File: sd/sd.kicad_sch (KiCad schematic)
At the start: 34 parts, among them J1 Micro_SD_Card_Det2, J3 STM32WORLD_BOARD, J4 STM32WORLD_CONNECTOR_1, J5 STM32WORLD_CONNECTOR_2

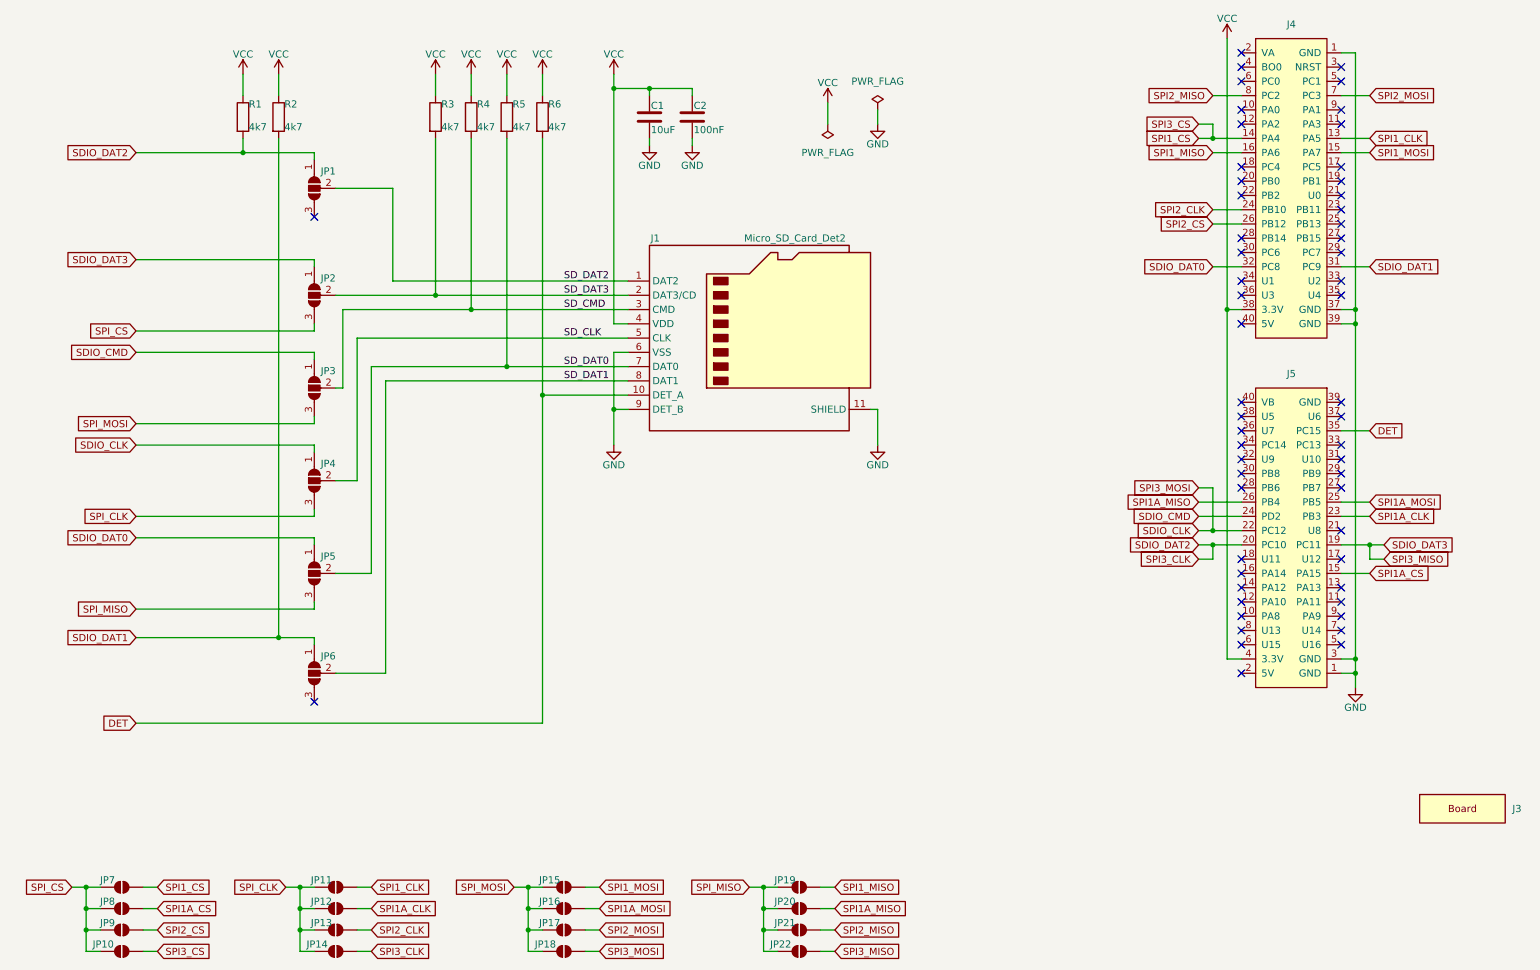
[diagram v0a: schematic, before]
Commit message: Ordered sd rev a
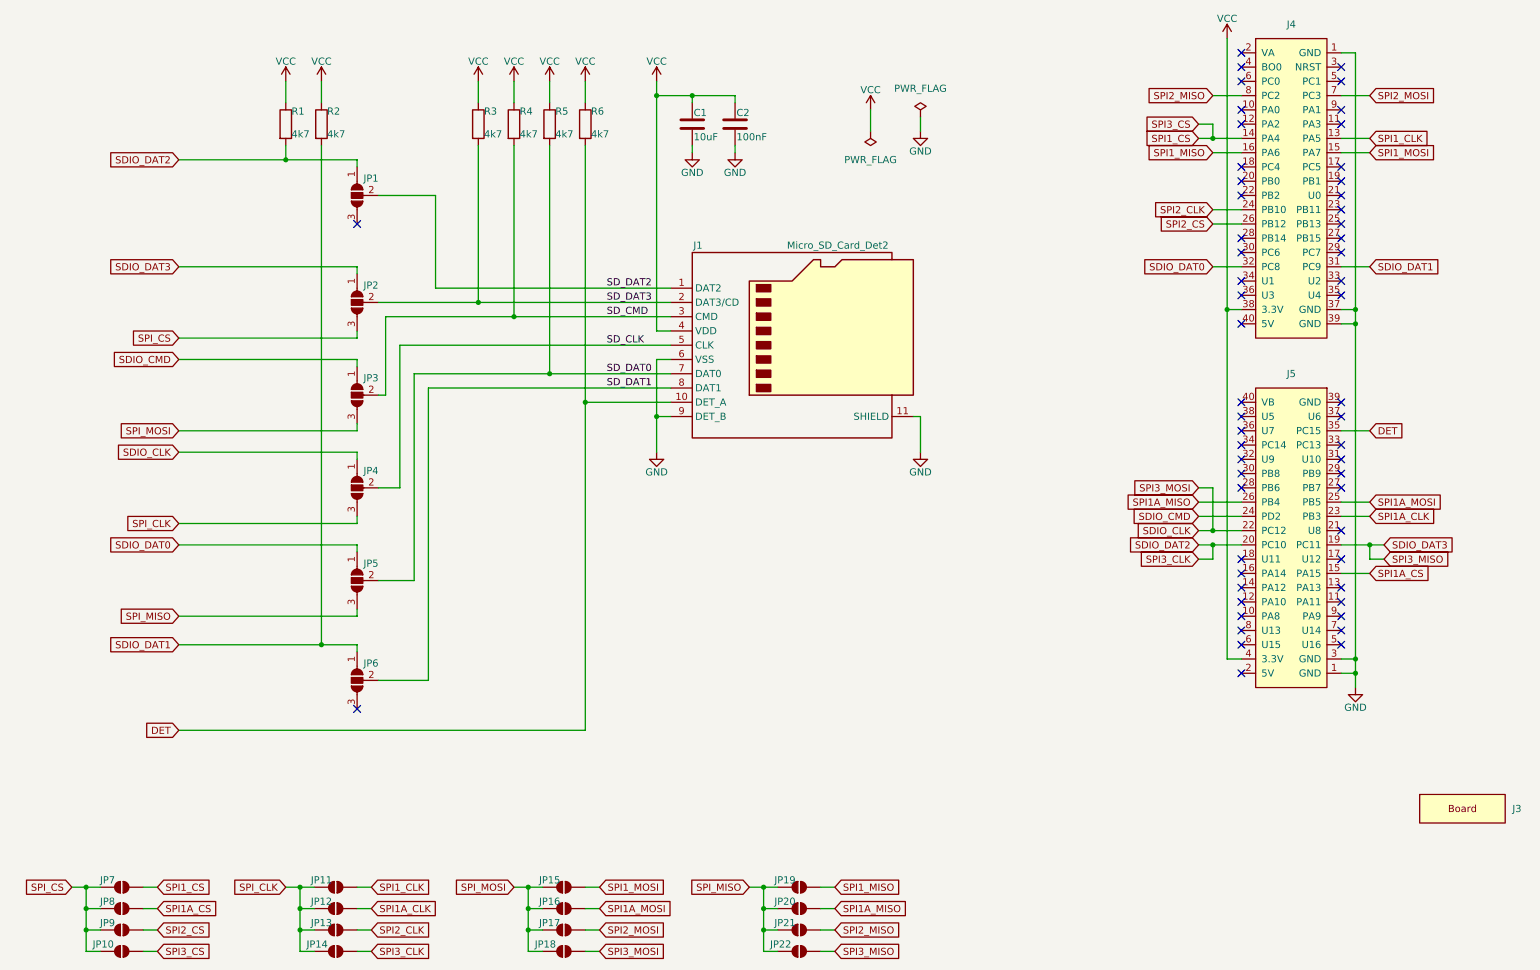
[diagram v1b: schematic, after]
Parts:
- C1: LCSC C719027 -> C1588
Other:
- moved on the sheet: C1, C2, J1, JP1, JP2, JP3, JP4, JP5, JP6, R1, R2, R3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
